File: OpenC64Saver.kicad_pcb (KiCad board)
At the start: 2 copper layers, 23.2 x 52.1 mm, 17 parts, among them J1 Power I/O, Q1 PN2222A, Q2 PN2222A, X1 OSHW_LOGO, X2 SCREW_HOLE, X3 SCREW_HOLE

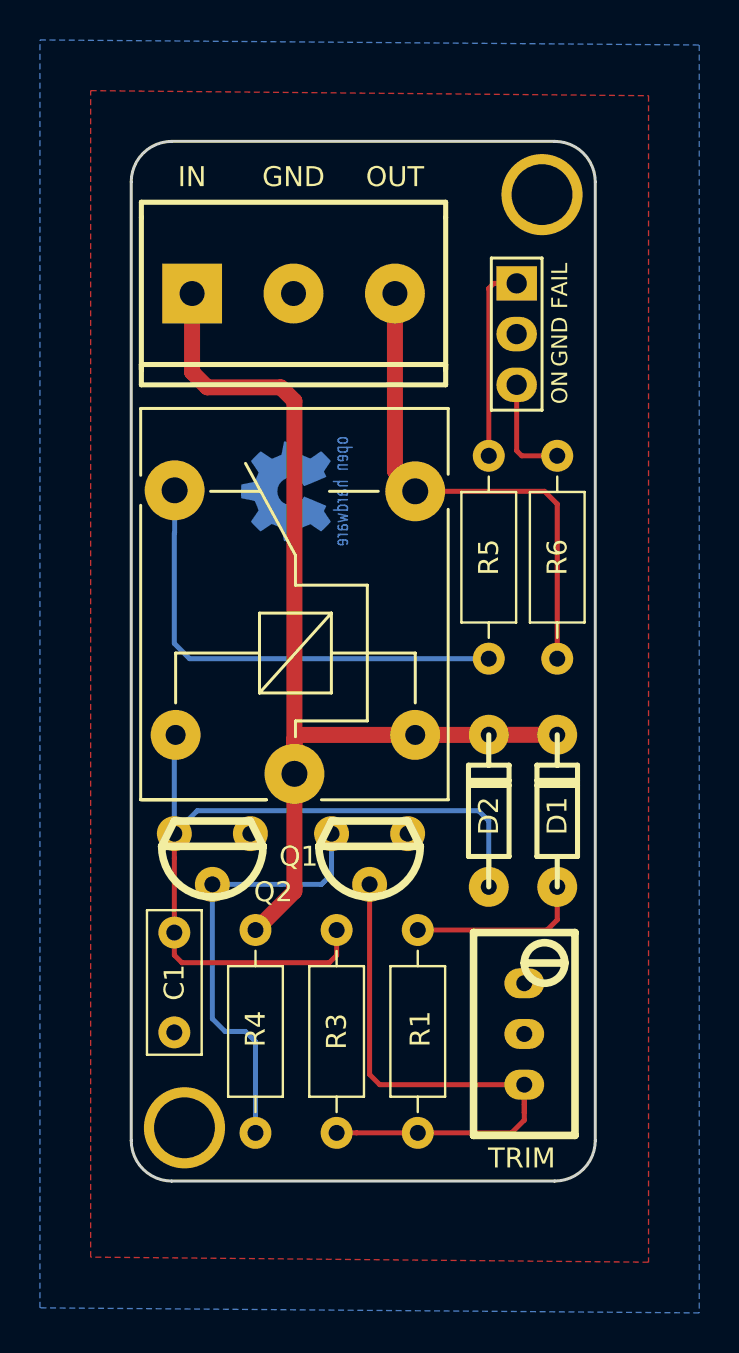
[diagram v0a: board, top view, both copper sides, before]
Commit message: Minor fix
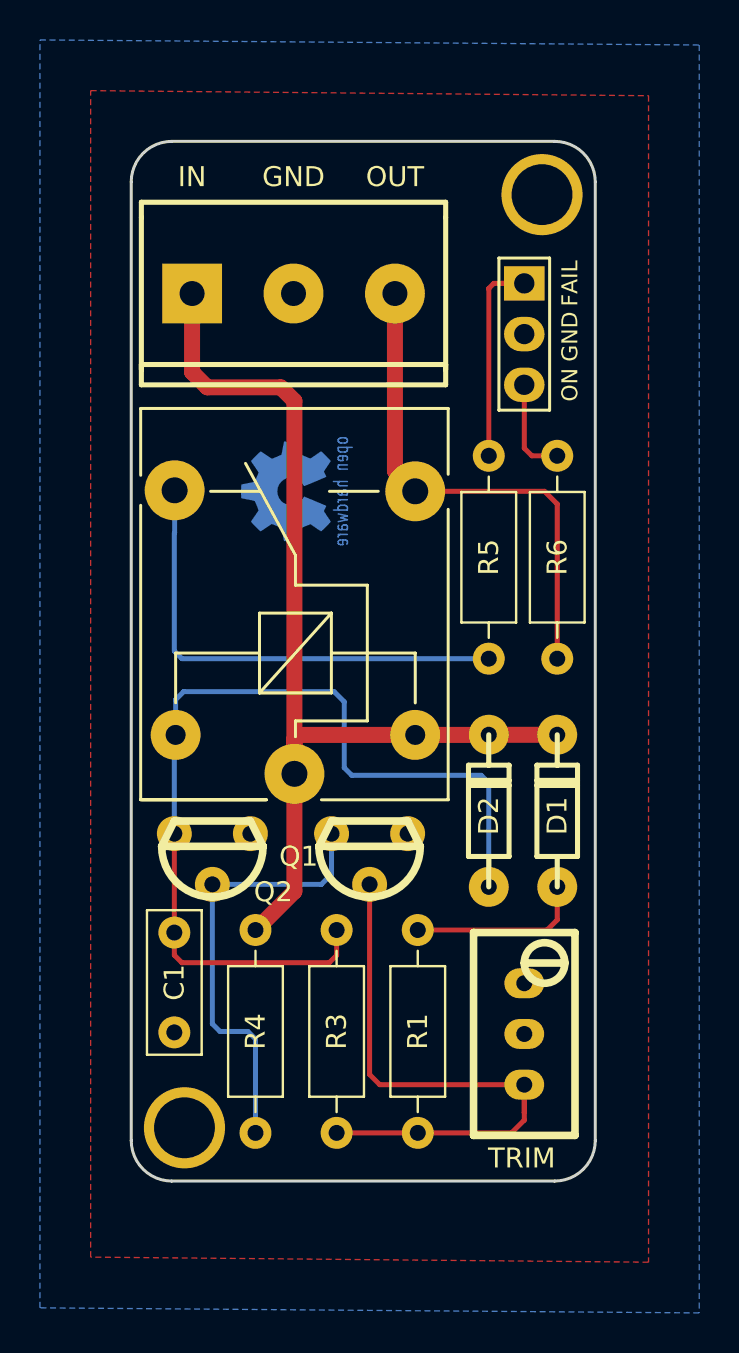
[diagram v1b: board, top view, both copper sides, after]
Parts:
- moved D3 0.38 mm to (156.3, 80.8)
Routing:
- net Net-(C1-Pad1): track 40.5 -> 47.4 mm
- net Net-(D3-Pad1): track 9.88 -> 11.0 mm
